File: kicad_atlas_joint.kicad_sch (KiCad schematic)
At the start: 33 parts, among them IC1 AS5600, J1 USB_OTG, J2 CONN1, J3 CONN2, J5 ARM_SWD_TC2030, SW1 RESET, U1 STM32F411CEUx, U2 LM2596S-3.3, U3 INA226, Y1 ACO-25MHz

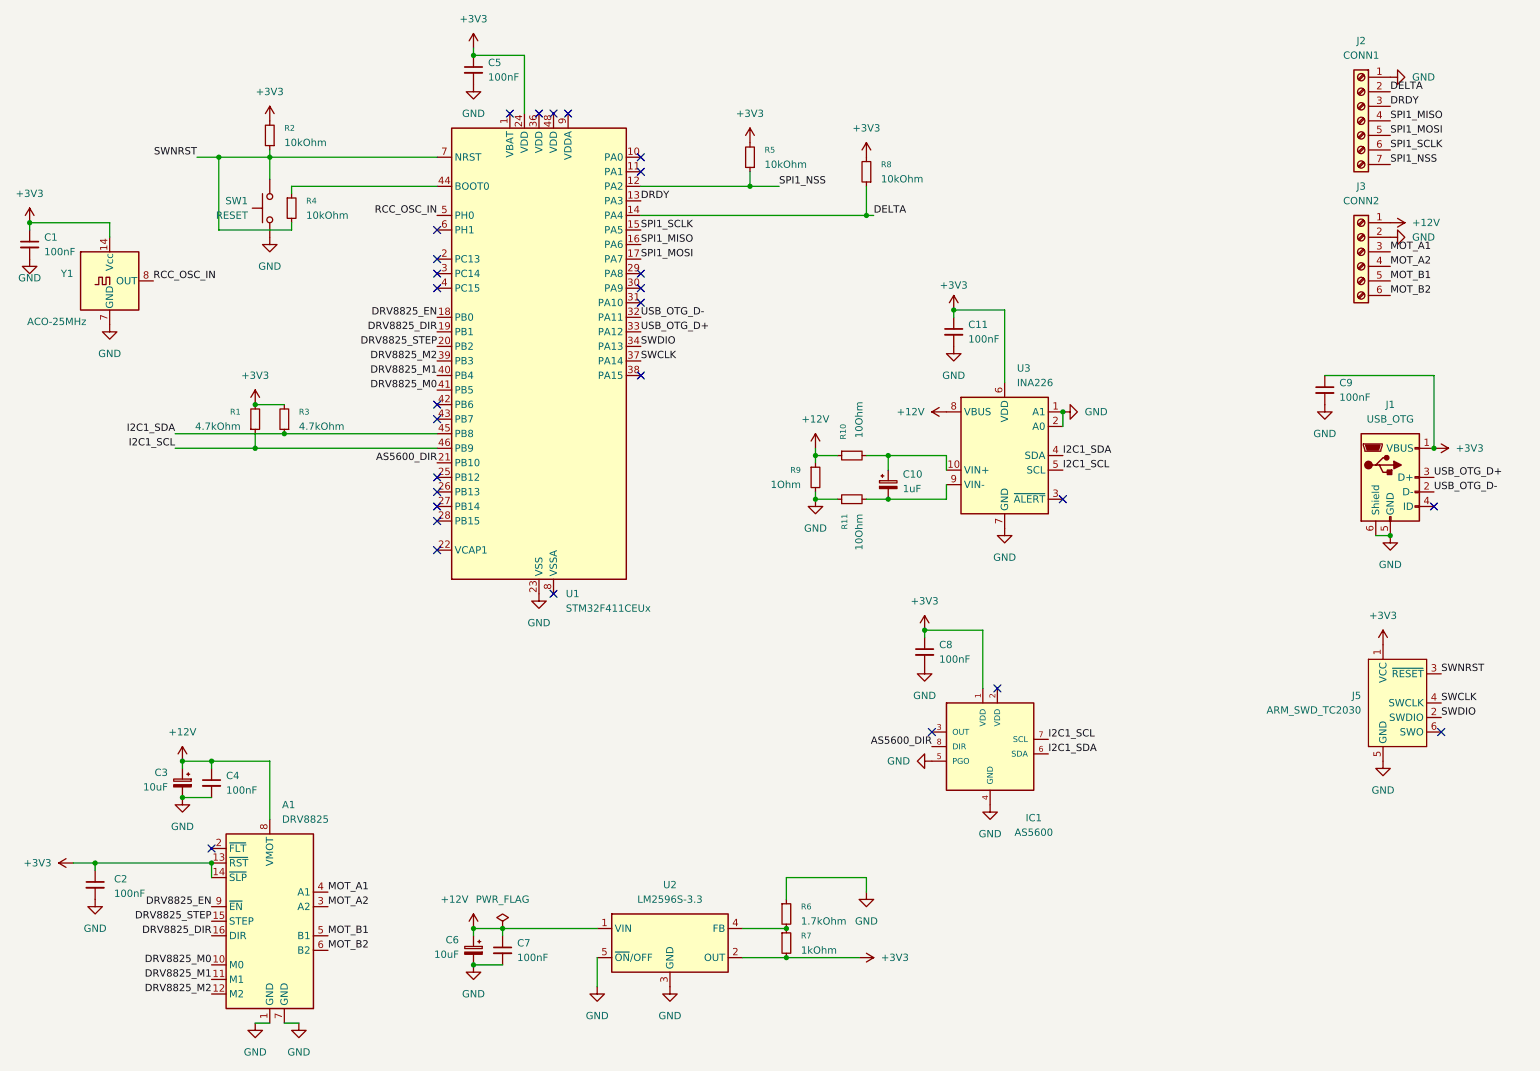
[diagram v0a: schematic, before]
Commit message: changes
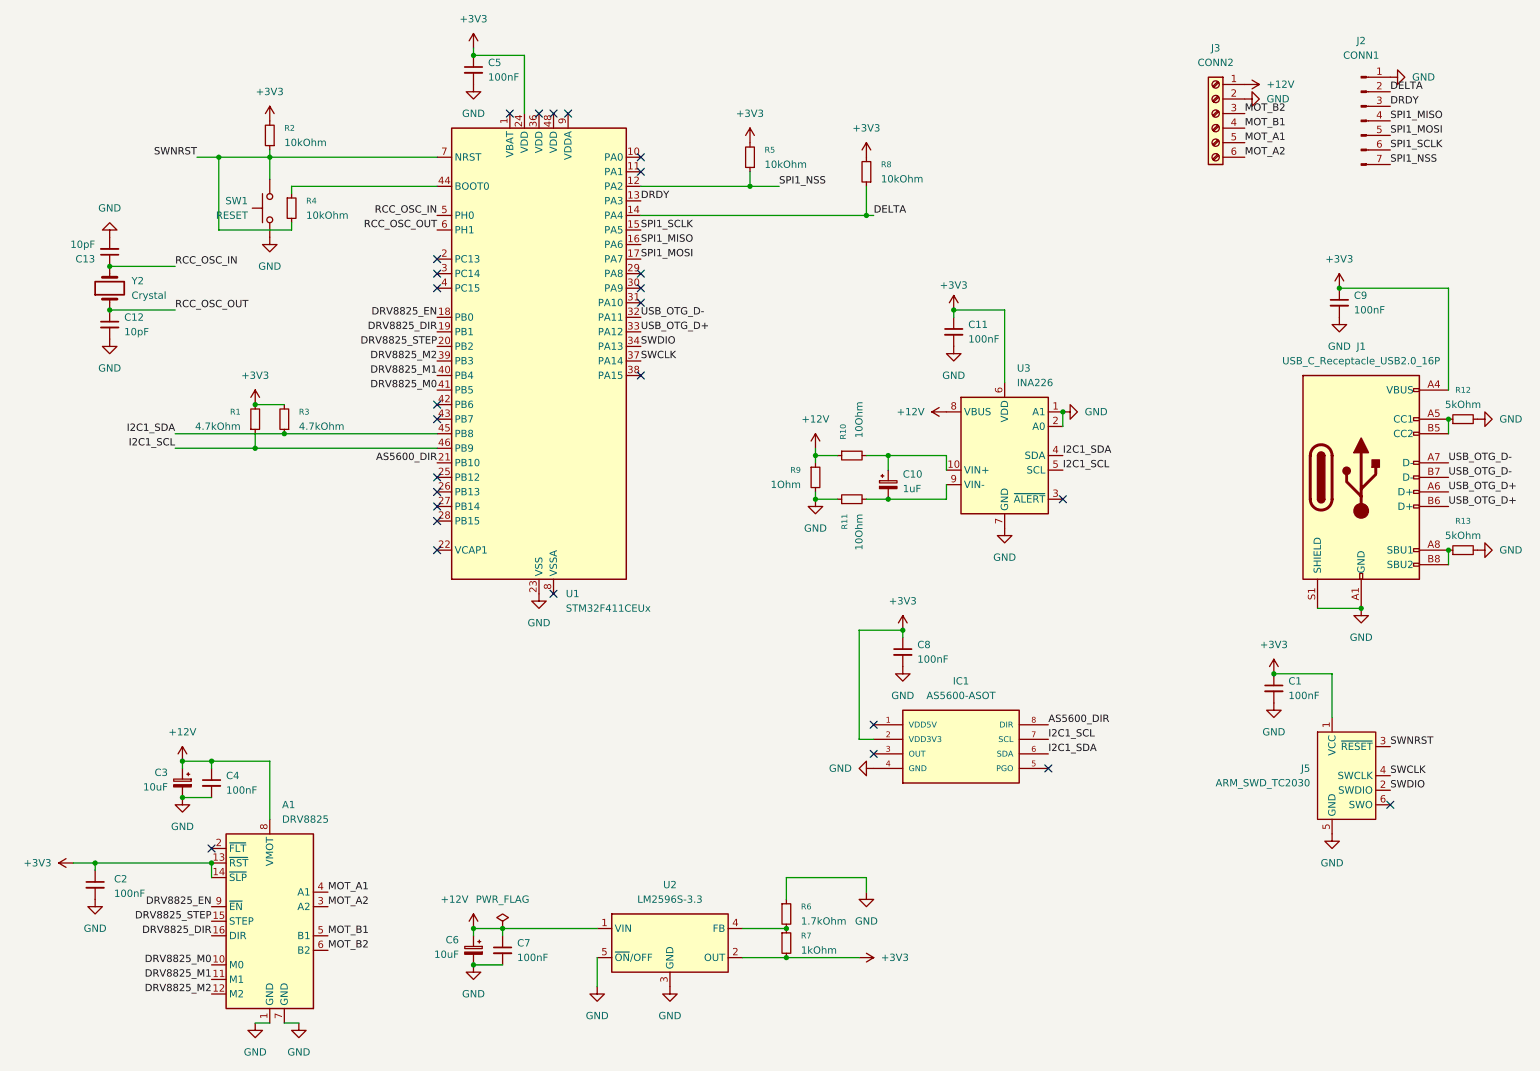
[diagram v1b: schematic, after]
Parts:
- removed J1: USB_OTG, symbol Connector:USB_OTG
- removed Y1: ACO-25MHz, Oscillator:Oscillator_DIP-14, symbol Oscillator:ACO-xxxMHz
- added C12, C13: 10pF, Capacitor_SMD:C_0201_0603Metric_Pad0.64x0.40mm_HandSolder, symbol Device:C_Small
- added J1: USB_C_Receptacle_USB2.0_16P, Connector_USB:USB_C_Receptacle_JAE_DX07S016JA1R1500, symbol Connector:USB_C_Receptacle_USB2.0_16P
- added R12, R13: 5kOhm, Resistor_SMD:R_0201_0603Metric, symbol Device:R_Small
- added Y2: Crystal, Crystal:Crystal_AT310_D3.0mm_L10.0mm_Horizontal, symbol Device:Crystal
- C1, C10, C11, C2, C3, C4, C5, C6, C7, C8, C9: footprint (none) -> Capacitor_SMD:C_0201_0603Metric_Pad0.64x0.40mm_HandSolder
- IC1: value AS5600 -> AS5600-ASOT; footprint AS5600-ASOT:SOIC127P600X175-8N -> as5600:SOIC127P600X175-8N
- J2: footprint (none) -> Connector_JST:JST_SHL_SM07B-SHLS-TF_1x07-1MP_P1.00mm_Horizontal; symbol Connector:Screw_Terminal_01x07 -> Connector:Conn_01x07_Pin
- J3: footprint (none) -> TerminalBlock:TerminalBlock_Xinya_XY308-2.54-6P_1x06_P2.54mm_Horizontal
- R1, R10, R11, R2, R3, R4, R5, R6, R7, R8, R9, SW1: footprint (none) -> Resistor_SMD:R_0201_0603Metric
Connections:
- net +3V3: now also IC1.2 (VDD3V3), J1.A4 (VBUS), J1.A9 (VBUS), J1.B4 (VBUS), J1.B9 (VBUS); no longer IC1.1 (VDD)
- net GND: now also C12.2, C13.2, J1.A1 (GND), J1.A12 (GND), J1.B1 (GND), J1.B12 (GND), J1.S1 (SHIELD), R12.2, R13.2; no longer IC1.5 (PGO)
- net MOT_A1: now also J3.5 (Pin_5); no longer J3.3 (Pin_3)
- net MOT_A2: now also J3.6 (Pin_6); no longer J3.4 (Pin_4)
- net MOT_B1: now also J3.4 (Pin_4); no longer J3.5 (Pin_5)
- net MOT_B2: now also J3.3 (Pin_3); no longer J3.6 (Pin_6)
- net RCC_OSC_IN: now also C13.1, Y2.2
- net USB_OTG_D+: now also J1.A6 (D+), J1.B6 (D+)
- net USB_OTG_D-: now also J1.A7 (D-), J1.B7 (D-)
- net RCC_OSC_OUT: now reaches U1.6 (PH1)
- net RCC_OSC_OUT: now also C12.1, Y2.1
- new net: J1.A8 (SBU1), J1.B8 (SBU2), R13.1
- new net: J1.A5 (CC1), J1.B5 (CC2), R12.1
- no-connect marks 28 -> 27
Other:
- moved on the sheet: C8, C9, J3, J5
